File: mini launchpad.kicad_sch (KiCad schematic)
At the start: 110 parts, among them P1 USB_C_Plug_USB2.0, SW65 SW_DPDT_x2, SW66 RotaryEncoder_Switch_MP, SW67 RotaryEncoder_Switch_MP, SW68 RotaryEncoder_Switch_MP, SW69 RotaryEncoder_Switch_MP, SW70 RotaryEncoder_Switch_MP, SW71 RotaryEncoder_Switch_MP, SW72 RotaryEncoder_Switch_MP, SW73 RotaryEncoder_Switch_MP, SW74 SW_Push, SW75 SW_Push, U1 MCP23017_ML, U10 W25Q128JVS, U11 MCP23017_ML, U2 MCP23017_ML, U3 MCP23017_ML, U4 MCP23017_ML, U5 CP2615-xx-xM, U6 TMUX1574PW, U7 CH334R, U8 RP2040, U9 NCP1117-3.3_TO252, Y1 12MHz

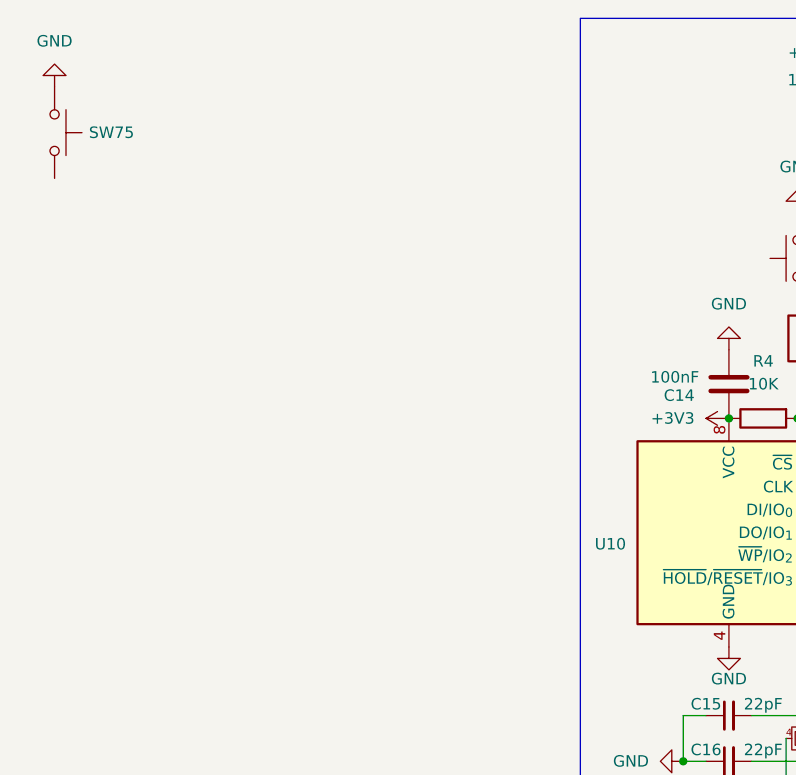
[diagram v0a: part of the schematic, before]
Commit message: pcb update
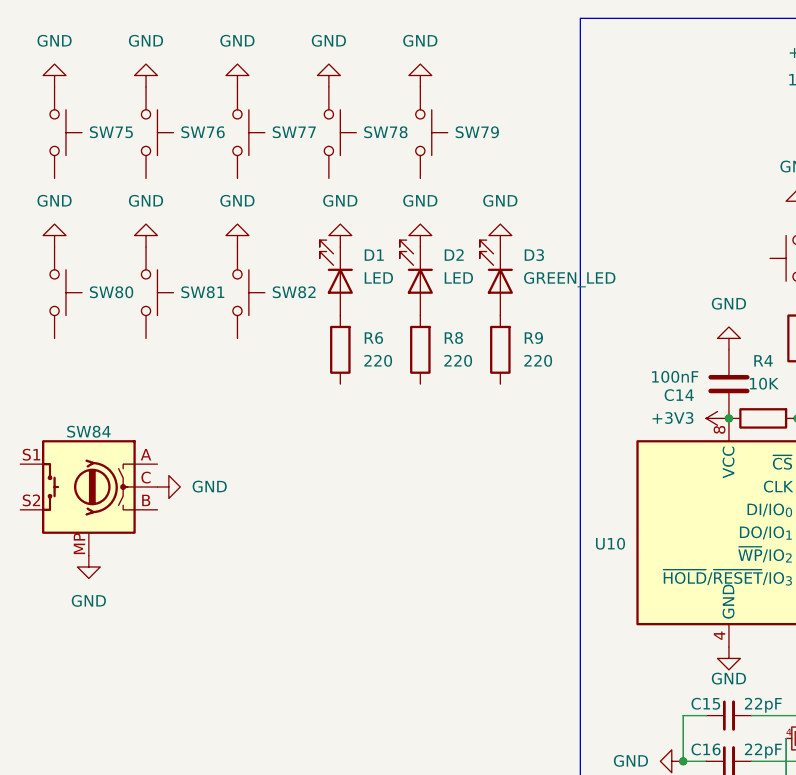
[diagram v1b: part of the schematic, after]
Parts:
- added D1, D2: LED, LED_SMD:LED_1206_3216Metric, symbol Device:LED
- added D3: GREEN_LED, LED_SMD:LED_1206_3216Metric, symbol Device:LED
- added R6, R8, R9: 220, Resistor_SMD:R_0402_1005Metric, symbol Device:R
- added SW76, SW77, SW78, SW79, SW80, SW81, SW82: SW_Push, Button_Switch_Keyboard:SW_Cherry_MX_1.00u_PCB, symbol Switch:SW_Push
- added SW84: RotaryEncoder_Switch_MP, Rotary_Encoder:RotaryEncoder_Alps_EC11E-Switch_Vertical_H20mm_MountingHoles, symbol Device:RotaryEncoder_Switch_MP
- SW74, SW75: footprint (none) -> Button_Switch_Keyboard:SW_Cherry_MX_1.00u_PCB
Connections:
- net GND: now also D1.1 (K), D2.1 (K), D3.1 (K), SW76.1, SW77.1, SW78.1, SW79.1, SW80.1, SW81.1, SW82.1, SW84.C, SW84.MP
- new net: D2.2 (A), R8.2
- new net: D1.2 (A), R6.2
- new net: D3.2 (A), R9.2

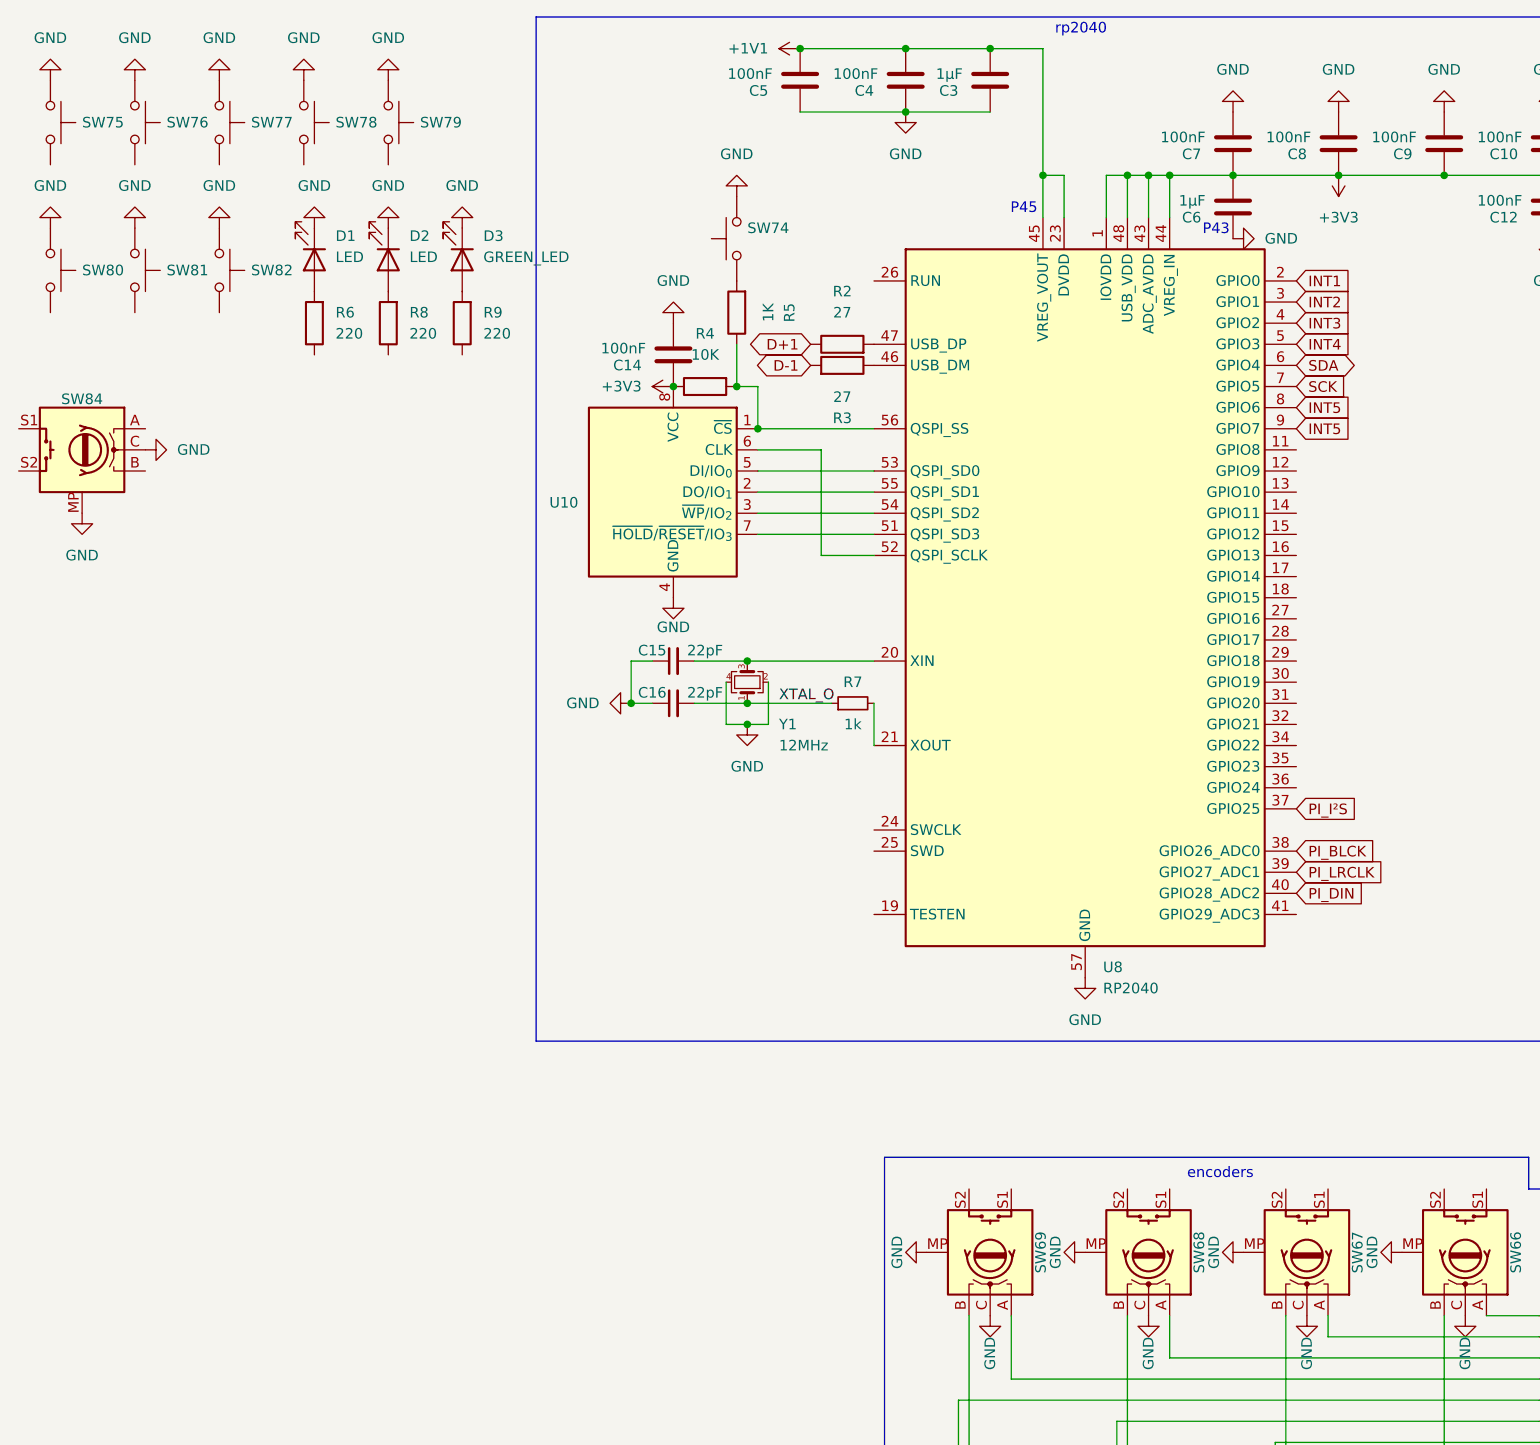
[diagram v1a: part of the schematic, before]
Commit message: pcb update
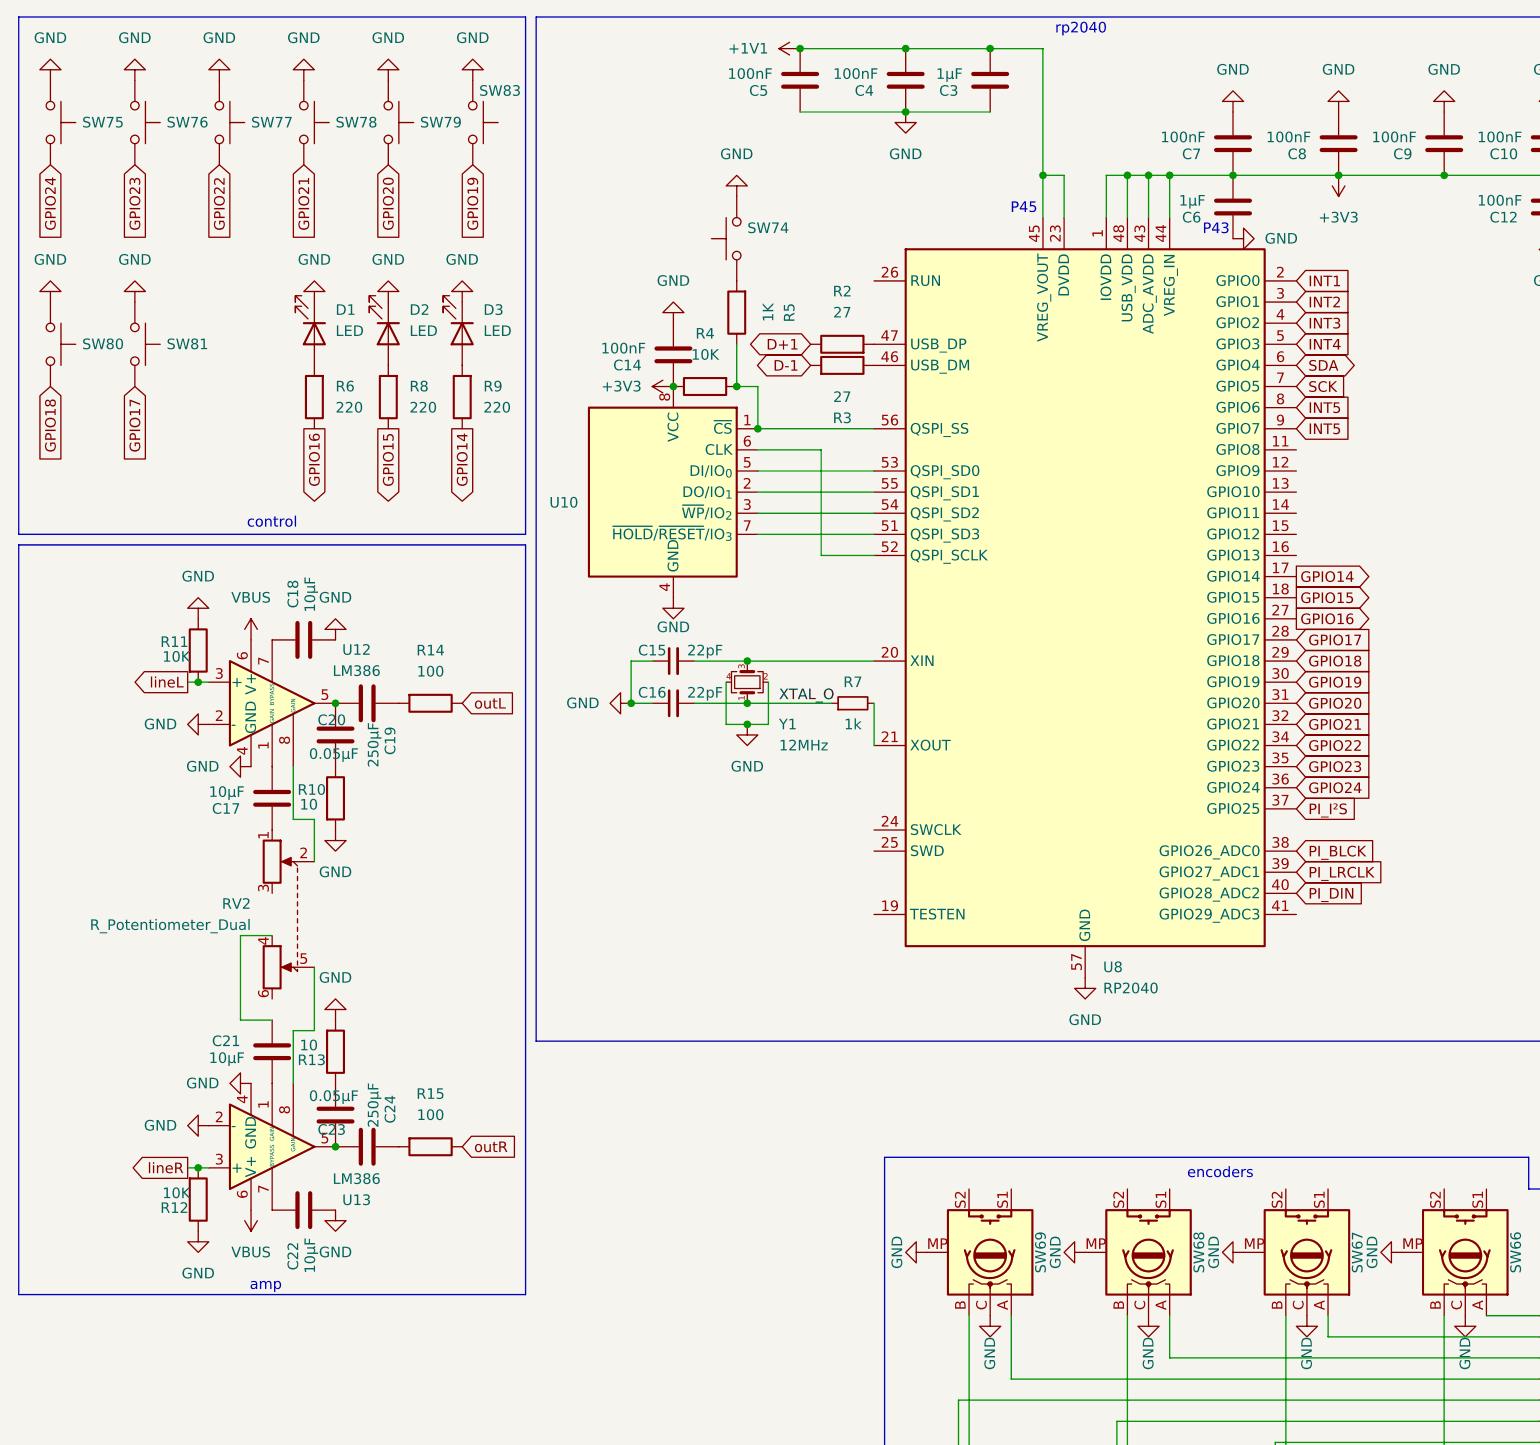
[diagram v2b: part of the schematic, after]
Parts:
- removed SW82: SW_Push, Button_Switch_Keyboard:SW_Cherry_MX_1.00u_PCB, symbol Switch:SW_Push
- removed SW84: RotaryEncoder_Switch_MP, Rotary_Encoder:RotaryEncoder_Alps_EC11E-Switch_Vertical_H20mm_MountingHoles, symbol Device:RotaryEncoder_Switch_MP
- added C17, C18, C21, C22: 10µF, Capacitor_SMD:C_0201_0603Metric, symbol Device:C
- added C19, C24: 250µF, Capacitor_SMD:C_0201_0603Metric, symbol Device:C
- added C20, C23: 0.05µF, Capacitor_SMD:C_0201_0603Metric, symbol Device:C
- added R10, R13: 10, Resistor_SMD:R_0402_1005Metric, symbol Device:R
- added R11, R12: 10K, Resistor_SMD:R_0402_1005Metric, symbol Device:R
- added R14, R15: 100, Resistor_SMD:R_0402_1005Metric, symbol Device:R
- added RV2: R_Potentiometer_Dual, Potentiometer_THT:Potentiometer_Alpha_RD902F-40-00D_Dual_Vertical, symbol Device:R_Potentiometer_Dual
- added SW83: SW_Push, Button_Switch_Keyboard:SW_Cherry_MX_1.00u_PCB, symbol Switch:SW_Push
- added U12, U13: LM386, Package_DIP:DIP-8_W7.62mm_Socket, symbol Amplifier_Audio:LM386
- D3: value GREEN_LED -> LED
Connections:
- net GND: now also C18.1, C22.1, R10.2, R11.1, R12.1, R13.2, SW83.1, U12.2 (-), U12.4 (GND), U13.2 (-), U13.4 (GND)
- net VBUS: now also U12.6 (V+), U13.6 (V+)
- net GPIO20: now reaches SW79.2
- net GPIO20: now also U8.31 (GPIO20)
- net GPIO16: now reaches R6.1
- net GPIO16: now also U8.27 (GPIO16)
- net GPIO18: now reaches SW80.2
- net GPIO18: now also U8.29 (GPIO18)
- net GPIO14: now reaches R9.1
- net GPIO14: now also U8.17 (GPIO14)
- net GPIO24: now reaches SW75.2
- net GPIO24: now also U8.36 (GPIO24)
- net GPIO21: now reaches SW78.2
- net GPIO21: now also U8.32 (GPIO21)
- net GPIO15: now reaches U8.18 (GPIO15)
- net GPIO15: now also R8.1
- net GPIO17: now reaches U8.28 (GPIO17)
- net GPIO17: now also SW81.2
- net GPIO19: now reaches U8.30 (GPIO19)
- net GPIO19: now also SW83.2
- net GPIO22: now reaches U8.34 (GPIO22)
- net GPIO22: now also SW77.2
- net GPIO23: now reaches U8.35 (GPIO23)
- net GPIO23: now also SW76.2
- new net: C17.1, U12.1 (GAIN)
- new net: C19.1, C20.1, U12.5
- new net: C18.2, U12.7 (BYPASS)
- new net: RV2.2, U12.8 (GAIN)
- new net: C22.2, U13.7 (BYPASS)
- new net: C23.1, C24.1, U13.5
- new net: C24.2, R15.2
- new net: C23.2, R13.1
- new net: C19.2, R14.2
- new net: C20.2, R10.1
- new net: C17.2, RV2.1
- new net: C21.1, U13.1 (GAIN)
- new net: RV2.5, U13.8 (GAIN)
- new net: C21.2, RV2.4
- new net lineL: R11.2, U12.3 (+)
- new net lineR: R12.2, U13.3 (+)
- new net outL: R14.1
- new net outR: R15.1
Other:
- note added: "amp"
- note added: "control"
- moved on the sheet: D1, D2, D3, R6, R8, R9, SW80, SW81
